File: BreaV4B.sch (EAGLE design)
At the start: 32 parts, among them J1 XF2L-0535-1, J2 XF2L-0535-1, Q3 ABM-16MHZ, SW1 ESE31L11T, SW2 EVQ11U09K, SW3 LS12T2-T, U1 TPS62200, X1 22-23-2021

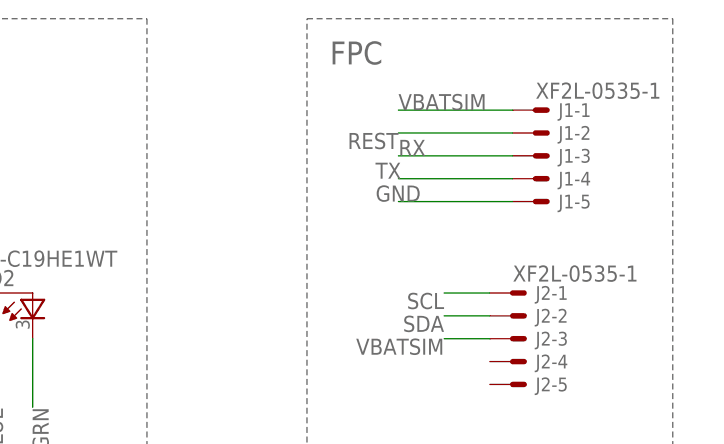
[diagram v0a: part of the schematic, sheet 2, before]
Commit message: Rx Tx
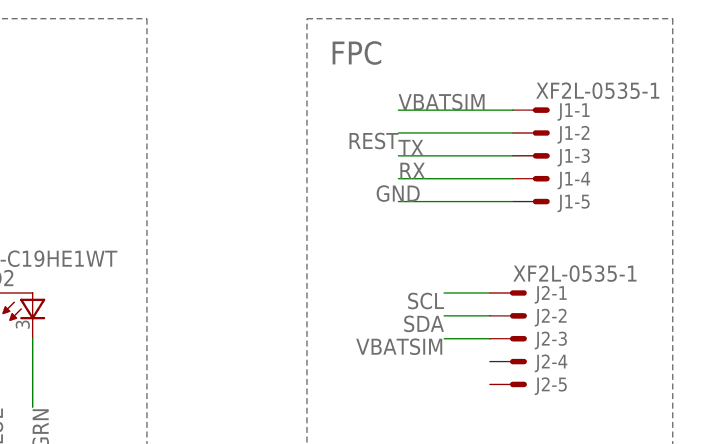
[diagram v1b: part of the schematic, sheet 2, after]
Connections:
- net RX: now also J1-4.MS; no longer J1-3.MS
- net TX: now also J1-3.MS; no longer J1-4.MS
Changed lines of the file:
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@@
-</segment>
-</net>
-<net name="RX" class="0">
-<segment>
-<pinref part="J1" gate="-3" pin="MS"/>
-<wire x1="160.02" y1="93.98" x2="147.32" y2="93.98" width="0.1524" layer="91"/>
-<label x="147.32" y="93.98" size="1.778" layer="95"/>
-</segment>
-</net>
-<net name="TX" class="0">
-<segment>
-<pinref part="J1" gate="-4" pin="MS"/>
-<wire x1="160.02" y1="91.44" x2="147.32" y2="91.44" width="0.1524" layer="91"/>
-<label x="144.78" y="91.44" size="1.778" layer="95"/>
 </segment>
 </net>
@@
 </segment>
 </net>
+<net name="RX" class="0">
+<segment>
+<pinref part="J1" gate="-4" pin="MS"/>
+<wire x1="160.02" y1="91.44" x2="147.32" y2="91.44" width="0.1524" layer="91"/>
+<label x="147.32" y="91.44" size="1.778" layer="95"/>
+</segment>
+</net>
+<net name="TX" class="0">
+<segment>
+<pinref part="J1" gate="-3" pin="MS"/>
+<wire x1="160.02" y1="93.98" x2="147.32" y2="93.98" width="0.1524" layer="91"/>
+<label x="147.32" y="93.98" size="1.778" layer="95"/>
+</segment>
+</net>
